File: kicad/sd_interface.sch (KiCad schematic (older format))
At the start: 4 parts, among them J1801 Screw_Terminal_01x06, J1802 Screw_Terminal_01x06, U1801 SI8661BD, U1802 SI8661BD

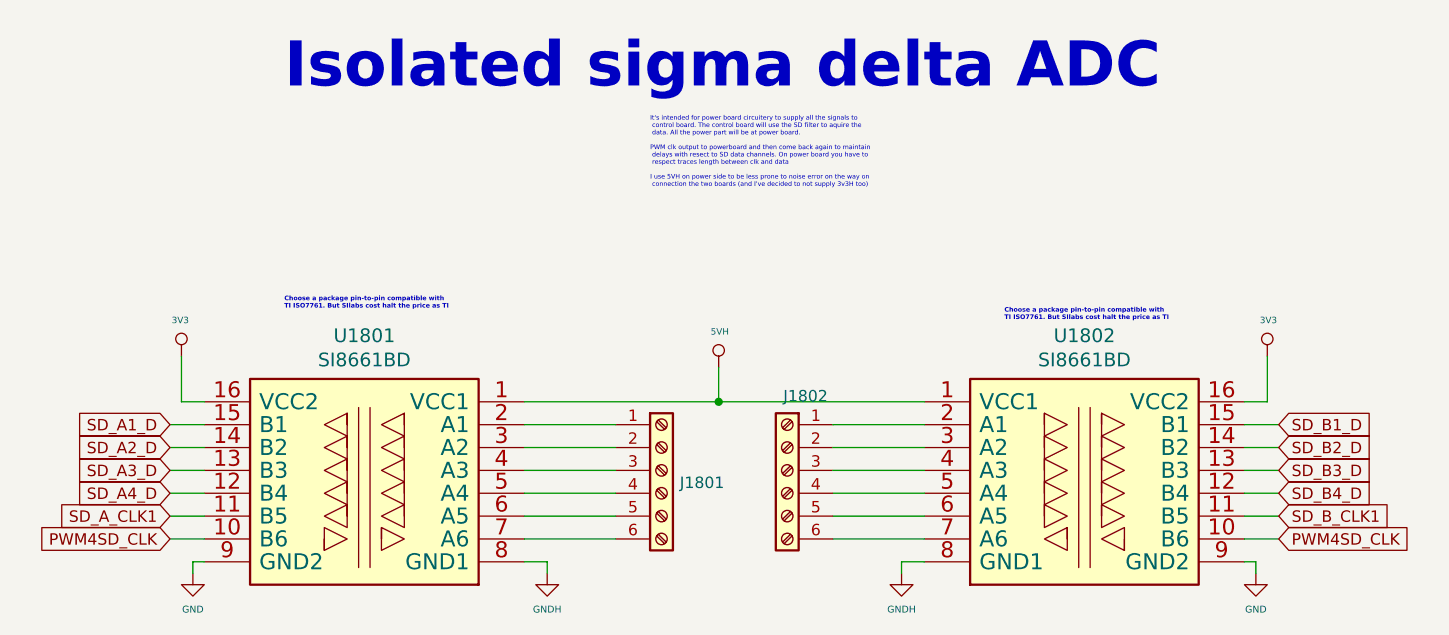
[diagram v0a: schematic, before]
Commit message: begin PCB!! it's amess but IT IS
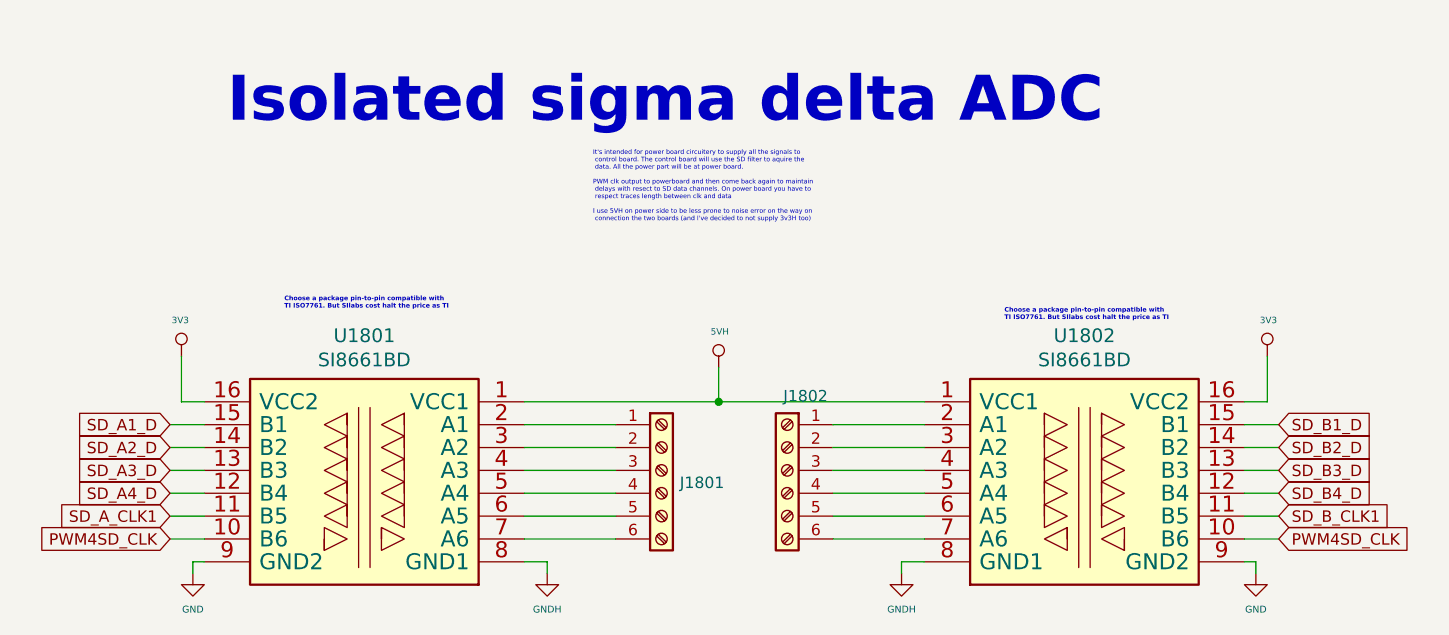
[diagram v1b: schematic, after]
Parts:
- J1801, J1802: footprint (none) -> Connector_PinHeader_2.54mm:PinHeader_1x06_P2.54mm_Vertical
- U1801, U1802: footprint (none) -> Package_SO:SOIC-16W_7.5x10.3mm_P1.27mm
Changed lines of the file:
@@
 Comment4 ""
 $EndDescr
-Text Notes 5450 1350 0    197  ~ 39
+Text Notes 5200 1500 0    197  ~ 39
 Isolated sigma delta ADC
 Text GLabel 9800 2800 2    50   Input ~ 0
@@
 F 0 "U1801" H 5800 3589 60  0000 C CNN
 F 1 "SI8661BD" H 5800 3483 60  0000 C CNN
-F 2 "" H 5200 3300 60  0000 C CNN
+F 2 "Package_SO:SOIC-16W_7.5x10.3mm_P1.27mm" H 5200 3300 60  0001 C CNN
 F 3 "../doc/datasheets/Si8660.pdf" H 5700 3600 60  0001 C CNN
 	1    5800 3000
@@
 F 0 "J1801" H 7180 2946 50  0000 L CNN
 F 1 "Screw_Terminal_01x06" H 7180 2901 50  0001 L CNN
-F 2 "" H 7100 3000 50  0001 C CNN
+F 2 "Connector_PinHeader_2.54mm:PinHeader_1x06_P2.54mm_Vertical" H 7100 3000 50  0001 C CNN
 F 3 "~" H 7100 3000 50  0001 C CNN
 	1    7100 3000
@@
 F 0 "U1802" H 8950 3589 60  0000 C CNN
 F 1 "SI8661BD" H 8950 3483 60  0000 C CNN
-F 2 "" H 8350 3300 60  0000 C CNN
+F 2 "Package_SO:SOIC-16W_7.5x10.3mm_P1.27mm" H 8350 3300 60  0001 C CNN
 F 3 "../doc/datasheets/Si8660.pdf" H 8850 3600 60  0001 C CNN
 	1    8950 3000
@@
 F 0 "J1802" H 7570 3325 50  0000 C CNN
 F 1 "Screw_Terminal_01x06" H 7730 2901 50  0001 L CNN
-F 2 "" H 7650 3000 50  0001 C CNN
+F 2 "Connector_PinHeader_2.54mm:PinHeader_1x06_P2.54mm_Vertical" H 7650 3000 50  0001 C CNN
 F 3 "~" H 7650 3000 50  0001 C CNN
 	1    7650 3000
@@
 Text Notes 8600 2350 0    20   ~ 4
 Choose a package pin-to-pin compatible with\nTI ISO7761. But SIlabs cost halt the price as TI
-Text Notes 7050 1800 0    20   ~ 0
+Text Notes 6800 1950 0    20   ~ 0
 It's intended for power board circuitery to supply all the signals to\n control board. The control board will use the SD filter to aquire the\n data. All the power part will be at power board.\n\nPWM clk output to powerboard and then come back again to maintain\n delays with resect to SD data channels. On power board you have to\n respect traces length between clk and data\n\nI use 5VH on power side to be less prone to noise error on the way on\n connection the two boards (and I've decided to not supply 3v3H too)\n\n
 $Comp
